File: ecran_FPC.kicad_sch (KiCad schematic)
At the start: 22 parts, among them J1 1-2328724-5, J6 MEC1-110-02-F-D-A, J8 MEC1-110-02-F-D-A, SW1 PEC11L-4220K-S0015

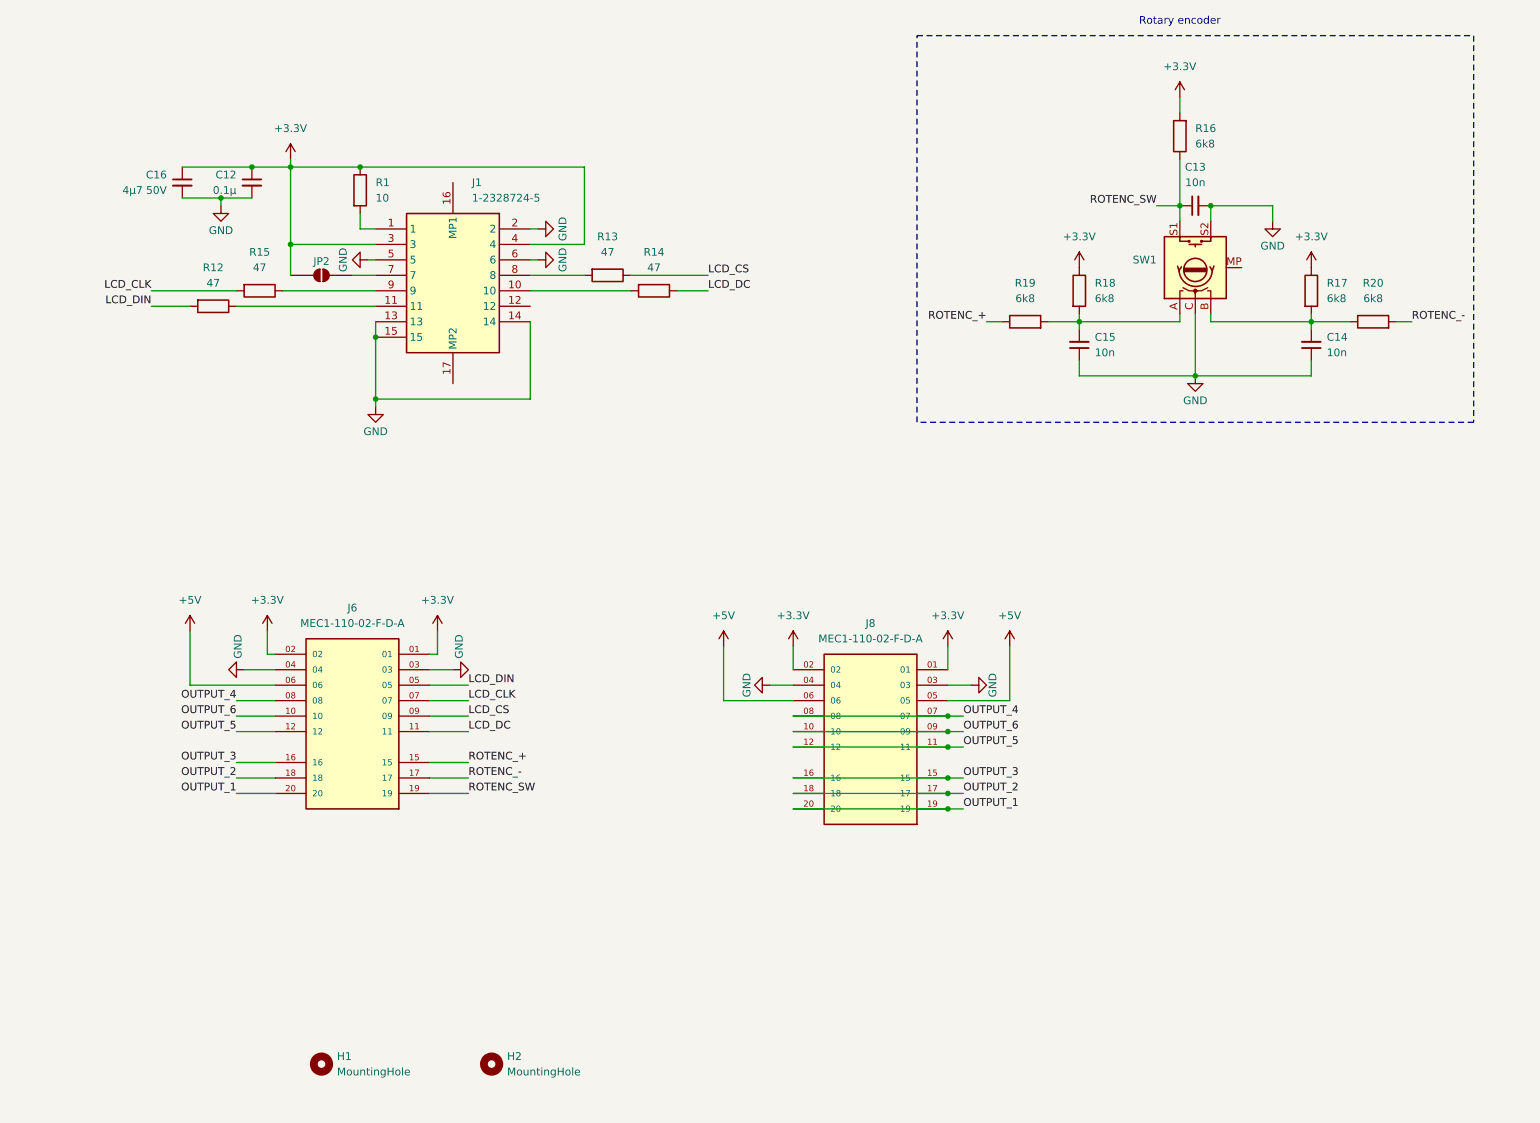
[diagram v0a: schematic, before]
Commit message: corrections
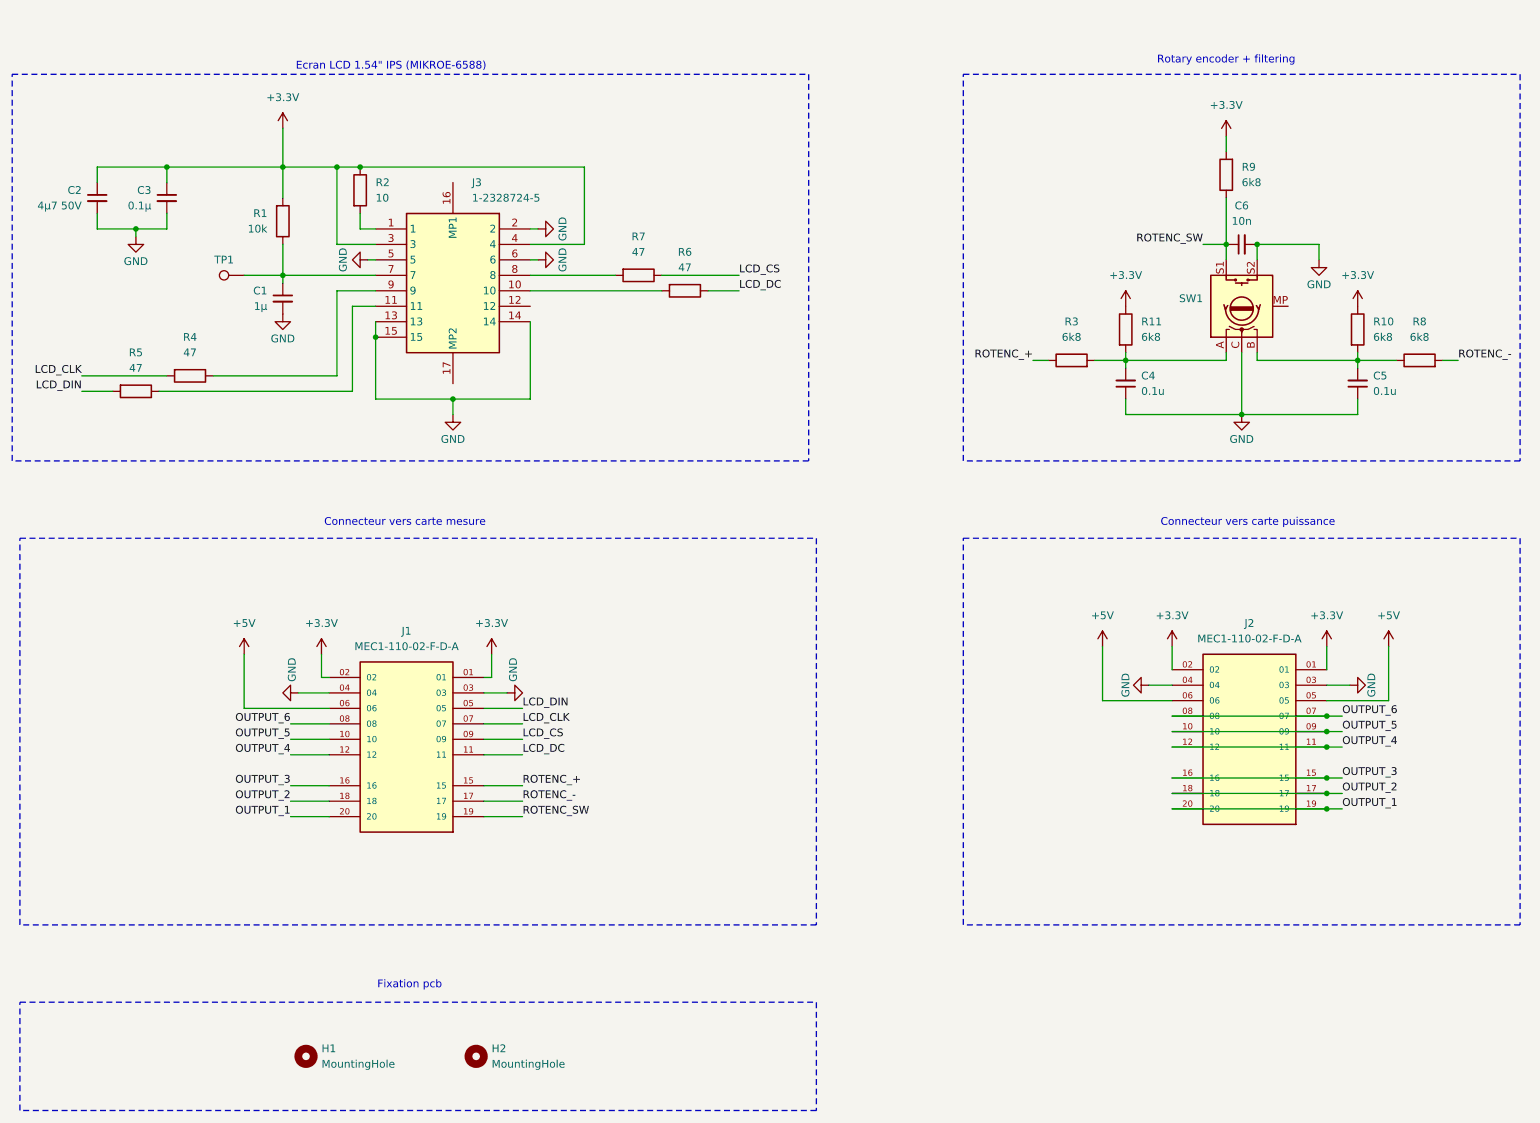
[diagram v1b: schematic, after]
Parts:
- removed JP2: SolderJumper_2_Open, Jumper:SolderJumper-2_P1.3mm_Open_RoundedPad1.0x1.5mm, symbol Jumper:SolderJumper_2_Open
- added C1: 1µ, Capacitor_SMD:C_0603_1608Metric_Pad1.08x0.95mm_HandSolder, symbol Device:C_Small
- added R1: 10k, Resistor_SMD:R_0603_1608Metric_Pad0.98x0.95mm_HandSolder, symbol Device:R
- added TP1: TestPoint, TestPoint:TestPoint_Pad_1.5x1.5mm, symbol Connector:TestPoint
- C4: renamed from C15; value 10n -> 0.1u; LCSC Part # C57112 -> C14663
- C5: renamed from C14; value 10n -> 0.1u; LCSC Part # C57112 -> C14663
- J3: renamed from J1; footprint 123287245 -> OPC:123287245
- SW1: footprint Rotary_Encoder:RotaryEncoder_Alps_EC11E-Switch_Vertical_H20mm_MountingHoles -> OPC:PEC11L4220KS0015
- renumbered C16 to C2, C12 to C3, C13 to C6, J6 to J1, J8 to J2, R17 to R10, R18 to R11, R1 to R2, R19 to R3, R15 to R4, R12 to R5, R14 to R6, R13 to R7, R20 to R8, R16 to R9
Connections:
- net +3.3V: now also R1.2
- net GND: now also C1.2
- net OUTPUT_4: now also J1.12, J2.11, J2.12; no longer J1.08, J2.07, J2.08
- net OUTPUT_5: now also J1.10, J2.09, J2.10; no longer J1.12, J2.11, J2.12
- net OUTPUT_6: now also J1.08, J2.07, J2.08; no longer J1.10, J2.09, J2.10
- net at J3.7: now also C1.1, R1.1, TP1.1
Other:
- note added: "Connecteur vers carte mesure"
- note added: "Connecteur vers carte puissance"
- note added: "Ecran LCD 1.54" IPS (MIKROE-6588)"
- note added: "Fixation pcb"
- note added: "Rotary encoder + filtering"
- note removed: "Rotary encoder"
- moved on the sheet: C2, C3, C4, C5, C6, H1, H2, J1, J2, R10, R11, R3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
